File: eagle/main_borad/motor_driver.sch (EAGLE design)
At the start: 11 parts, among them Q1 16Mhz, U1 ATMEGA8A-AU

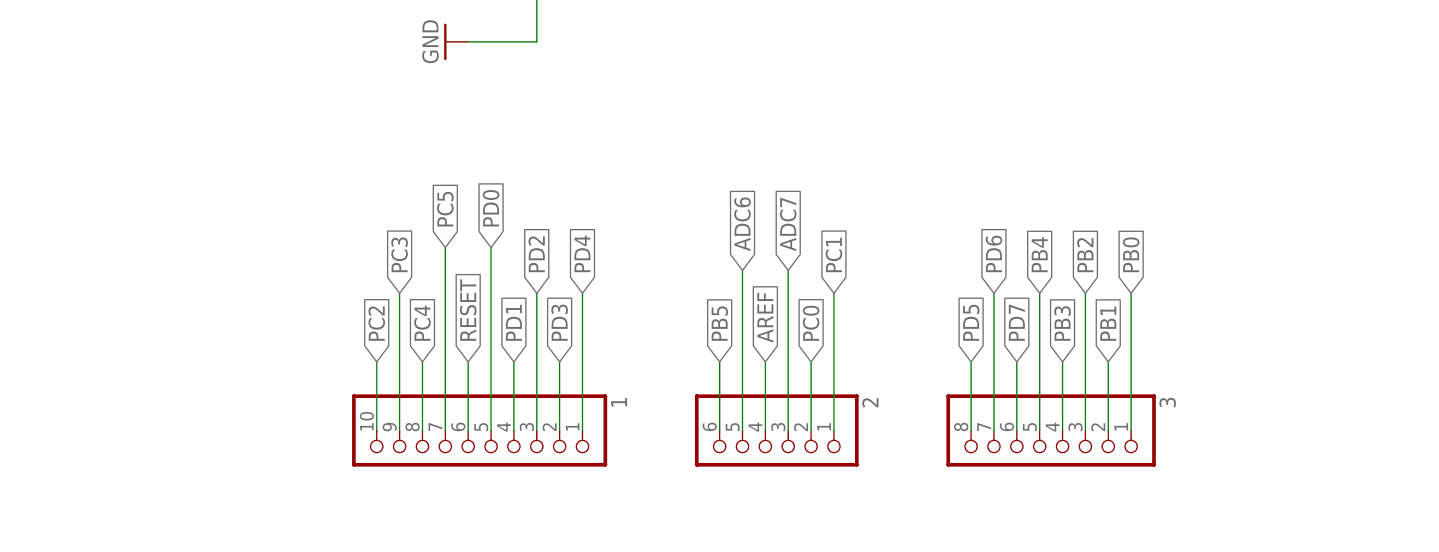
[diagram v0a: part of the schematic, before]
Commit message: mainborad shema - first version
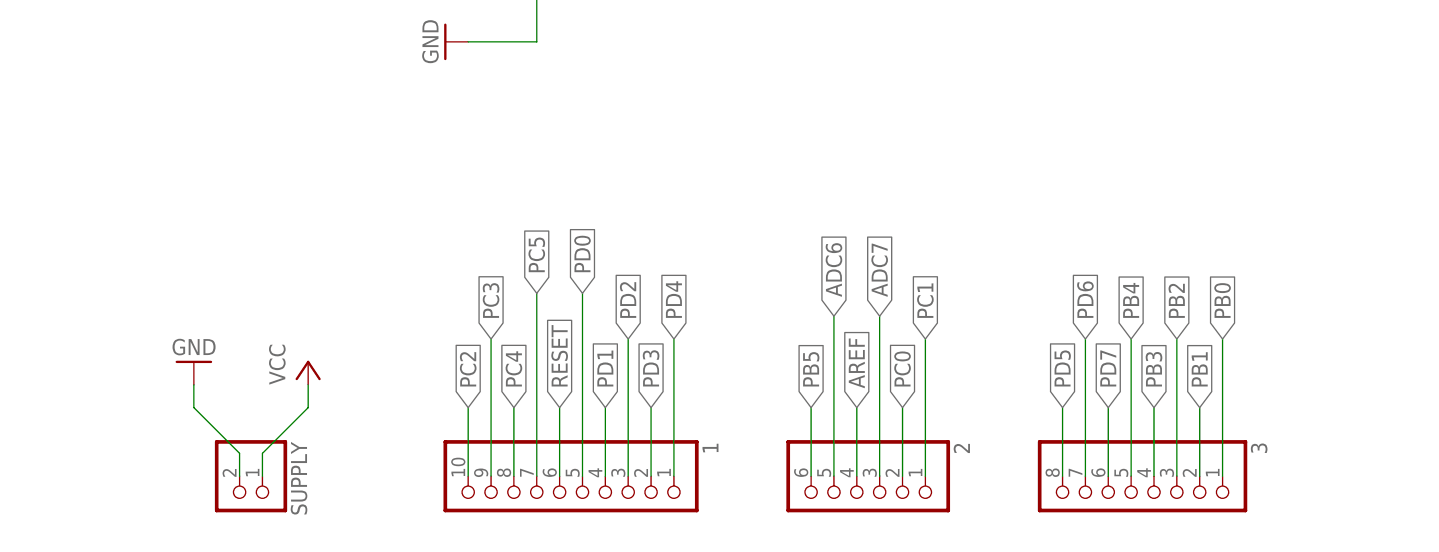
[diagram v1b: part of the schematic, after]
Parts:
- added SUPPLY: (no value), pinhead:PINHD-1X2
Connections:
- net GND: now also SUPPLY.2
- net VCC: now also SUPPLY.1
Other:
- moved on the sheet: 1, 2, 3

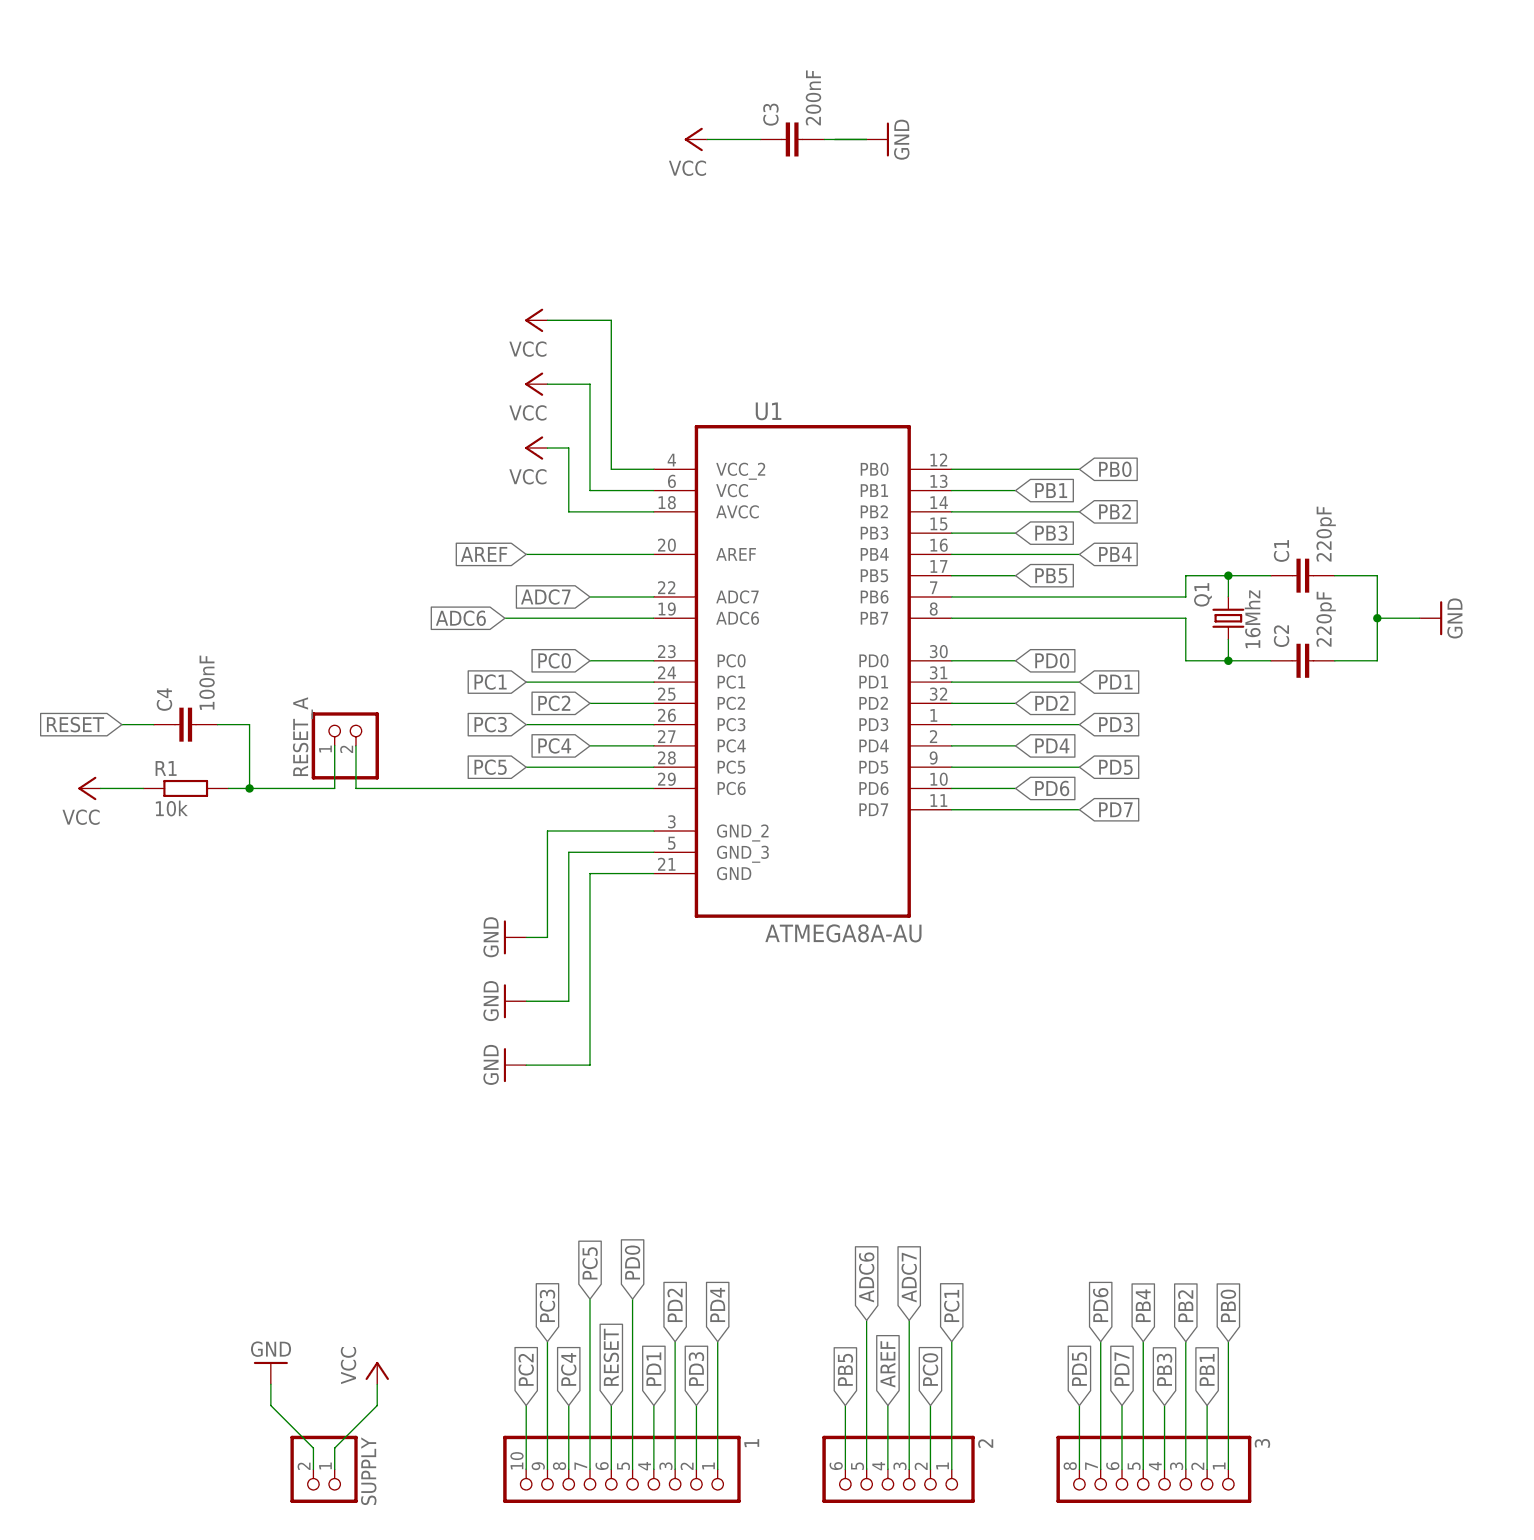
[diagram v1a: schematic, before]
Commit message: Druha verze navrhu desek pro rizeni podvozku.
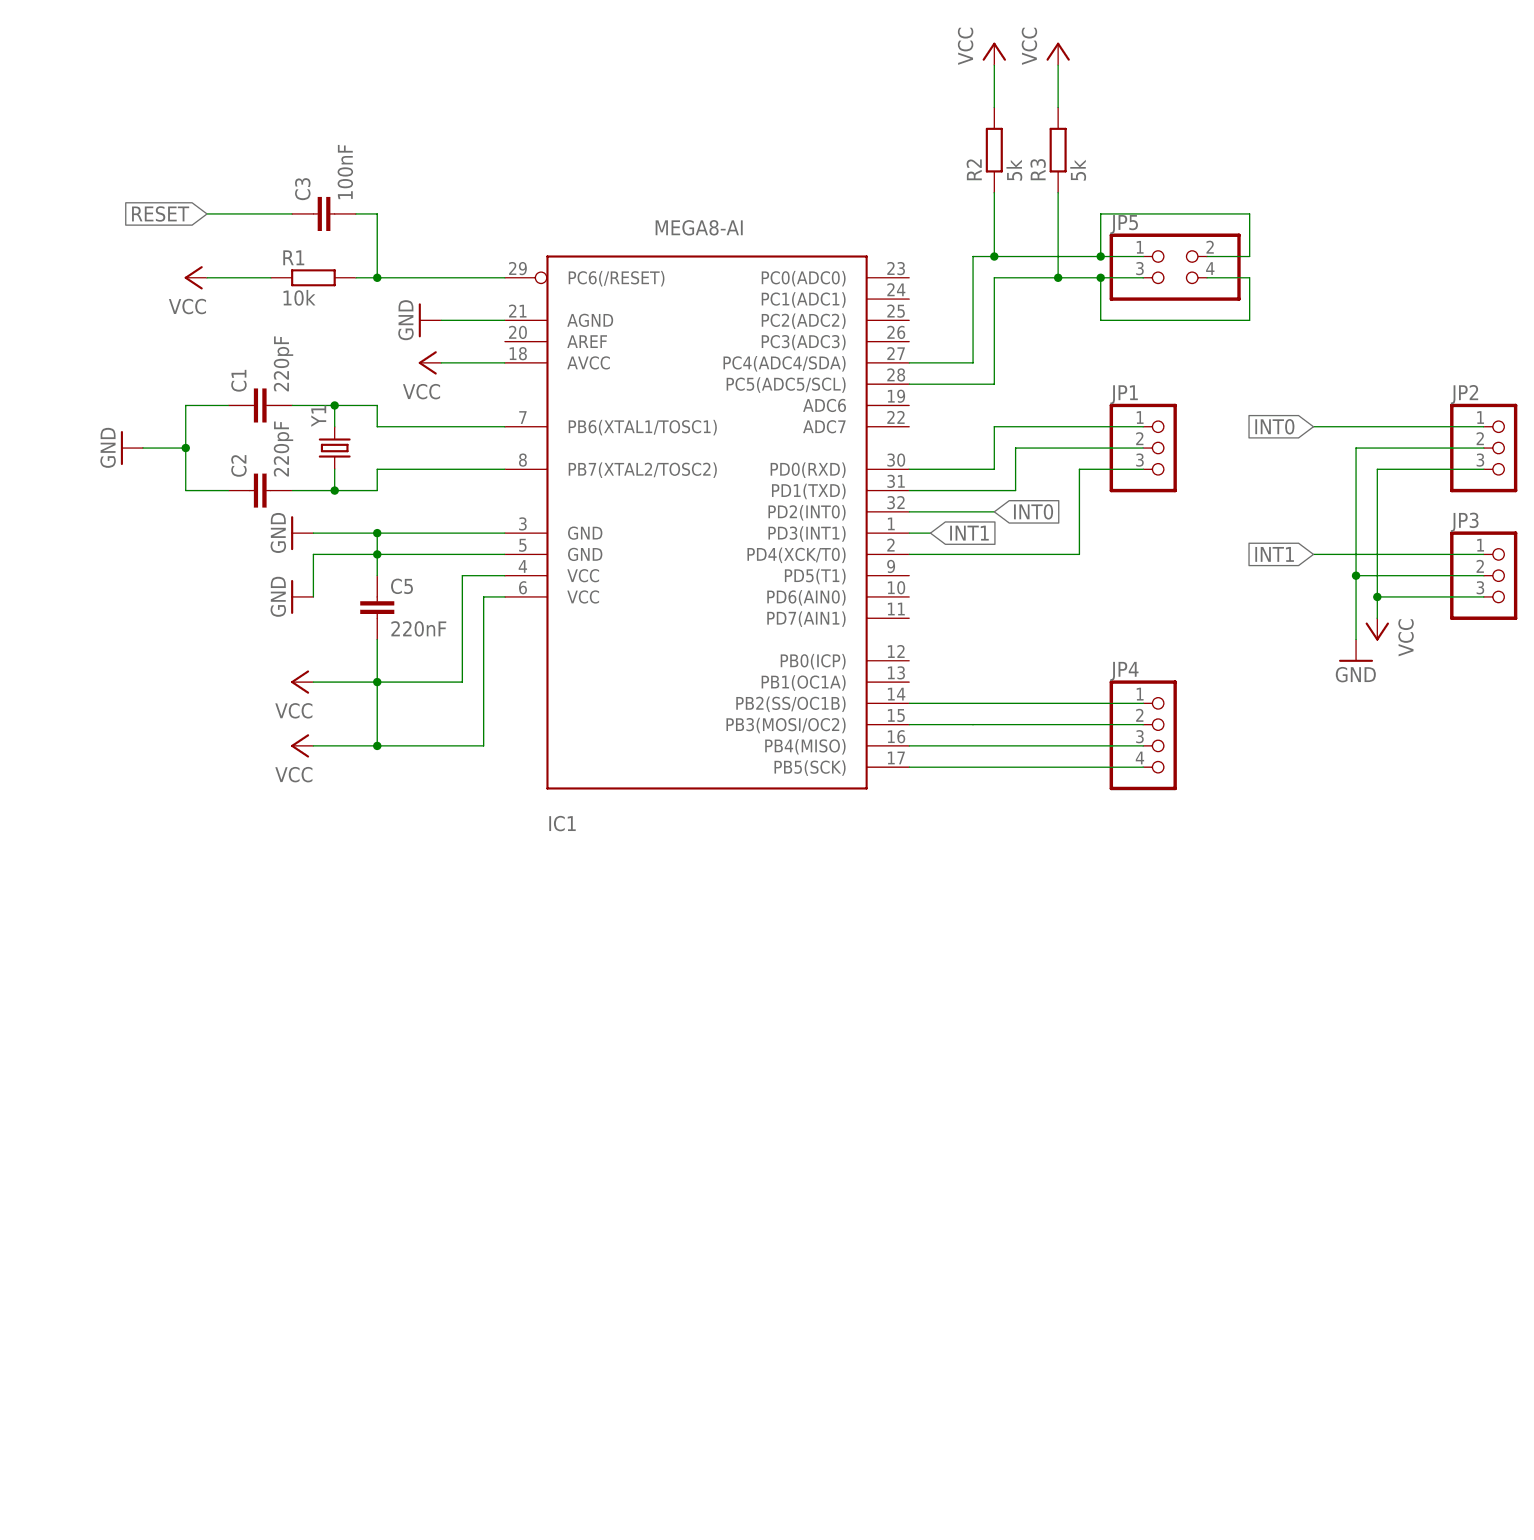
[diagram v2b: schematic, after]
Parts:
- removed 1: (no value), pinhead:PINHD-1X10
- removed 2: (no value), pinhead:PINHD-1X6
- removed 3: (no value), pinhead:PINHD-1X8
- removed C4: 100nF, capacitor-wima:C2,5-3
- removed Q1: 16Mhz, crystal:CRYSTALHC49U-V
- removed RESET_A, SUPPLY: (no value), pinhead:PINHD-1X2
- removed U1: ATMEGA8A-AU, Atmel_By_element14_Batch_1-00:ATMEGA8A-AU
- added C5: 220nF, SparkFun-Capacitors:CAP1206
- added IC1: MEGA8-AI, avr-7:MEGA8-AI
- added JP1, JP2, JP3: (no value), pinhead:PINHD-1X3
- added JP4: (no value), pinhead:PINHD-1X4
- added JP5: (no value), pinhead:PINHD-2X2
- added R2, R3: 5k, eagle-ltspice:RR1206
- added Y1: (no value), SparkFun-FreqCtrl:CRYSTALHC49US
- C1, C2: device capacitor-wima:C2,5-3 -> SparkFun-Capacitors:CAP1206
- C3: value 200nF -> 100nF; device capacitor-wima:C2,5-3 -> SparkFun-Capacitors:CAP1206
- R1: device eagle-ltspice:R -> eagle-ltspice:RR1206
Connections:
- removed net ADC6: 2.5, U1.ADC6
- removed net ADC7: 2.3, U1.ADC7
- removed net AREF: 2.4, U1.AREF
- removed net PB0: 3.1, U1.PB0
- removed net PB1: 3.2, U1.PB1
- removed net PB2: 3.3, U1.PB2
- removed net PB3: 3.4, U1.PB3
- removed net PB4: 3.5, U1.PB4
- removed net PB5: 2.6, U1.PB5
- removed net PC0: 2.2, U1.PC0
- removed net PC1: 2.1, U1.PC1
- removed net PC2: 1.10, U1.PC2
- removed net PC3: 1.9, U1.PC3
- removed net PC4: 1.8, U1.PC4
- removed net PC5: 1.7, U1.PC5
- removed net PD0: 1.5, U1.PD0
- removed net PD1: 1.4, U1.PD1
- removed net PD2: 1.3, U1.PD2
- removed net PD3: 1.2, U1.PD3
- removed net PD4: 1.1, U1.PD4
- removed net PD5: 3.8, U1.PD5
- removed net PD6: 3.7, U1.PD6
- removed net PD7: 3.6, U1.PD7
- removed net ^RESET: C4.2, R1.2, RESET_A.1
- new net INT0: IC1.PD2(INT0), JP2.1
- new net INT1: IC1.PD3(INT1), JP3.1
- new net N$10: IC1.PC4(ADC4/SDA), JP5.1, JP5.2, R2.1
- new net N$12: IC1.PB5(SCK), JP4.4
- new net N$13: IC1.PB4(MISO), JP4.3
- new net N$14: IC1.PB3(MOSI/OC2)
- new net N$15: IC1.PB2(SS/OC1B), JP4.1
- new net N$4: C3.2, IC1.PC6(/RESET), R1.2
- new net N$5: IC1.PD0(RXD), JP1.1
- new net N$6: IC1.PD4(XCK/T0), JP1.3
- new net N$7: JP4.2
- new net N$9: IC1.PC5(ADC5/SCL), JP5.3, JP5.4, R3.1
- net GND: now also C1.1, C2.1, C5.1, IC1.AGND, IC1.GND@1, IC1.GND@2, JP2.2, JP3.2; no longer C1.2, C2.2, C3.2, SUPPLY.2, U1.GND, U1.GND_2, U1.GND_3
- net N$1: now also IC1.PD1(TXD), JP1.2; no longer C1.1, Q1.2, U1.PB6
- net N$2: now also C2.2, IC1.PB7(XTAL2/TOSC2), Y1.1; no longer C2.1, Q1.1, U1.PB7
- net N$3: now also C1.2, IC1.PB6(XTAL1/TOSC1), Y1.2; no longer RESET_A.2, U1.PC6
- net RESET: now also C3.1; no longer 1.6, C4.1
- net VCC: now also C5.2, IC1.AVCC, IC1.VCC@1, IC1.VCC@2, JP2.3, JP3.3, R2.2, R3.2; no longer C3.1, SUPPLY.1, U1.AVCC, U1.VCC, U1.VCC_2
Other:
- moved on the sheet: C1, C2, C3, R1
